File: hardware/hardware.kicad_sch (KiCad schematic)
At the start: 21 parts, among them IC1 INA226AIDGST, IC2 E22-900M22S, IC3 INA226AIDGST, J1 BME280, J2 CJMCU-3935, U1 ESP32-C3_SUPERMINI, U2 DS3231SN, U3 CJMCU-3935, U4 FM24CL16B

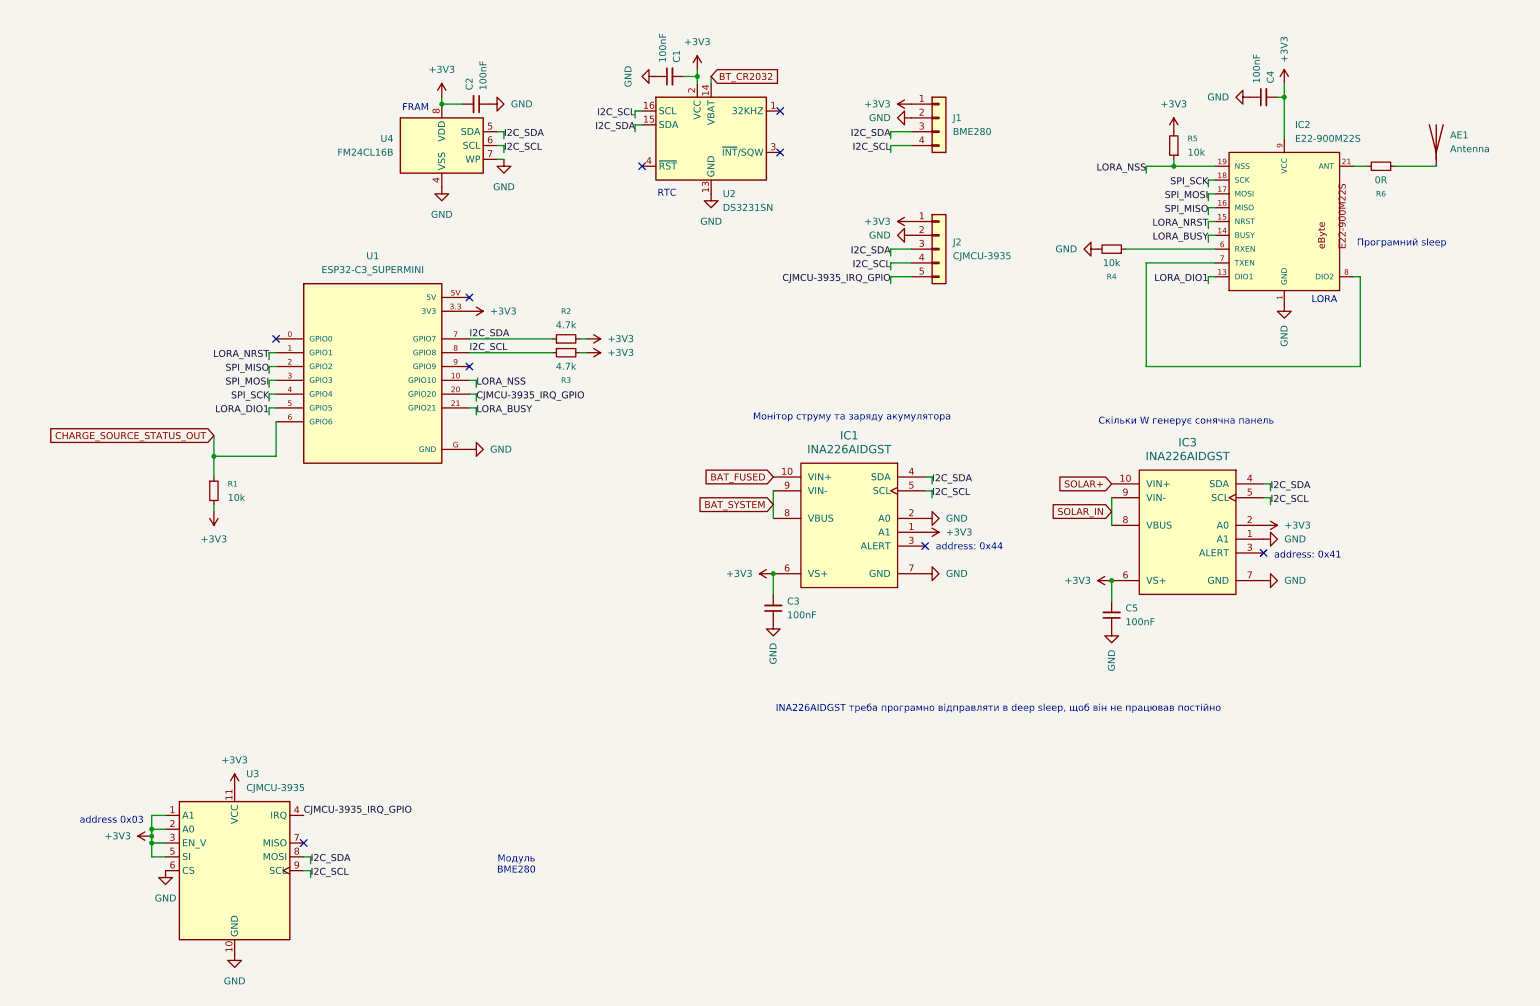
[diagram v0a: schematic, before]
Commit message: hardware improve i2c
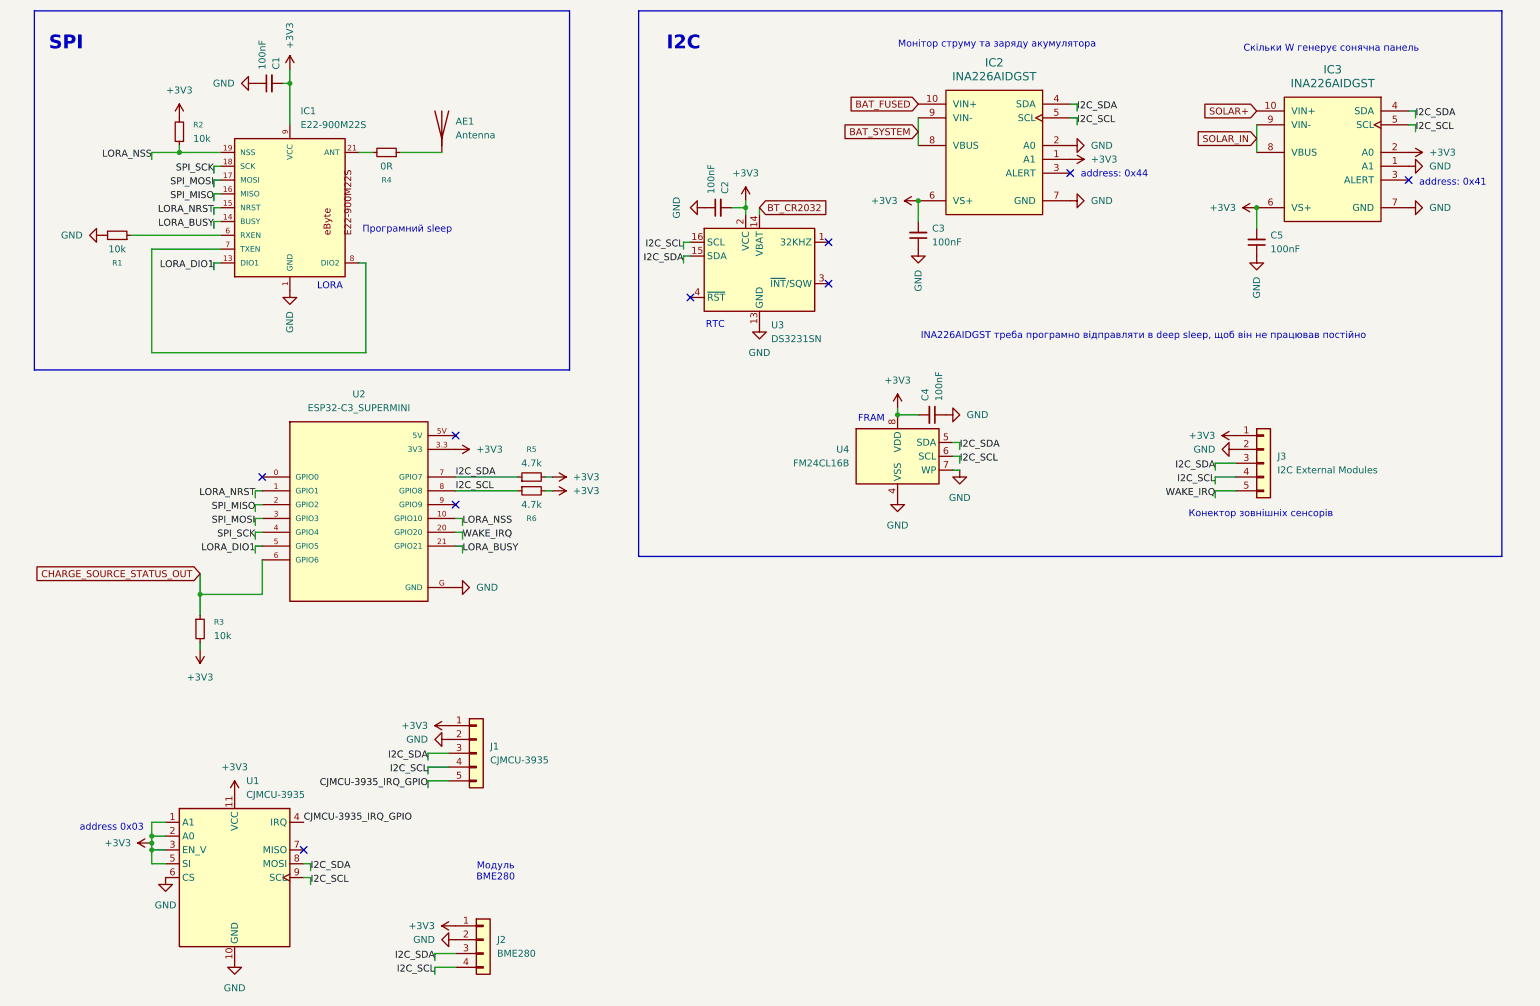
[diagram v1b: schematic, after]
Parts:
- removed J1: BME280, Connector_JST:JST_PH_B4B-PH-K_1x04_P2.00mm_Vertical, symbol Connector_Generic:Conn_01x04
- removed J2: CJMCU-3935, Connector_JST:JST_PH_B5B-PH-K_1x05_P2.00mm_Vertical, symbol Connector_Generic:Conn_01x05
- added J1: CJMCU-3935, Connector_JST:JST_PH_B5B-PH-K_1x05_P2.00mm_Vertical, symbol Connector_Generic:Conn_01x05
- added J2: BME280, Connector_JST:JST_PH_B4B-PH-K_1x04_P2.00mm_Vertical, symbol Connector_Generic:Conn_01x04
- added J3: I2C External Modules, Connector_JST:JST_PH_B5B-PH-K_1x05_P2.00mm_Vertical, symbol Connector_Generic:Conn_01x05
- renumbered C4 to C1, C1 to C2, C2 to C4, IC2 to IC1, IC1 to IC2, R4 to R1, R5 to R2, R1 to R3, R6 to R4, R2 to R5, R3 to R6, U3 to U1, U1 to U2, U2 to U3
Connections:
- net +3V3: now also J1.1 (Pin_1), J2.1 (Pin_1), J3.1 (Pin_1)
- net CJMCU-3935_IRQ_GPIO: now also J1.5 (Pin_5); no longer U2.20 (GPIO20)
- net GND: now also J1.2 (Pin_2), J2.2 (Pin_2), J3.2 (Pin_2)
- net I2C_SCL: now also J1.4 (Pin_4), J2.4 (Pin_4), J3.4 (Pin_4)
- net I2C_SDA: now also J1.3 (Pin_3), J2.3 (Pin_3), J3.3 (Pin_3)
- new net WAKE_IRQ: J3.5 (Pin_5), U2.20 (GPIO20)
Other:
- note added: "I2C"
- note added: "SPI"
- note added: "Конектор зовнішніх сенсорів"
- moved on the sheet: AE1, C1, C2, C3, C4, C5, IC1, IC2, IC3, R1, R2, R3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
